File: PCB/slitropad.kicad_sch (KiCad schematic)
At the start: 11 parts, among them SW1 SW_Push, SW2 SW_Push, SW3 SW_Push, SW4 SW_Push, SW5 SW_Push, SW6 SW_Push, SW7 SW_Push, SW8 SW_Push, SW9 SW_Push, U1 XIAO-RP2040-DIP

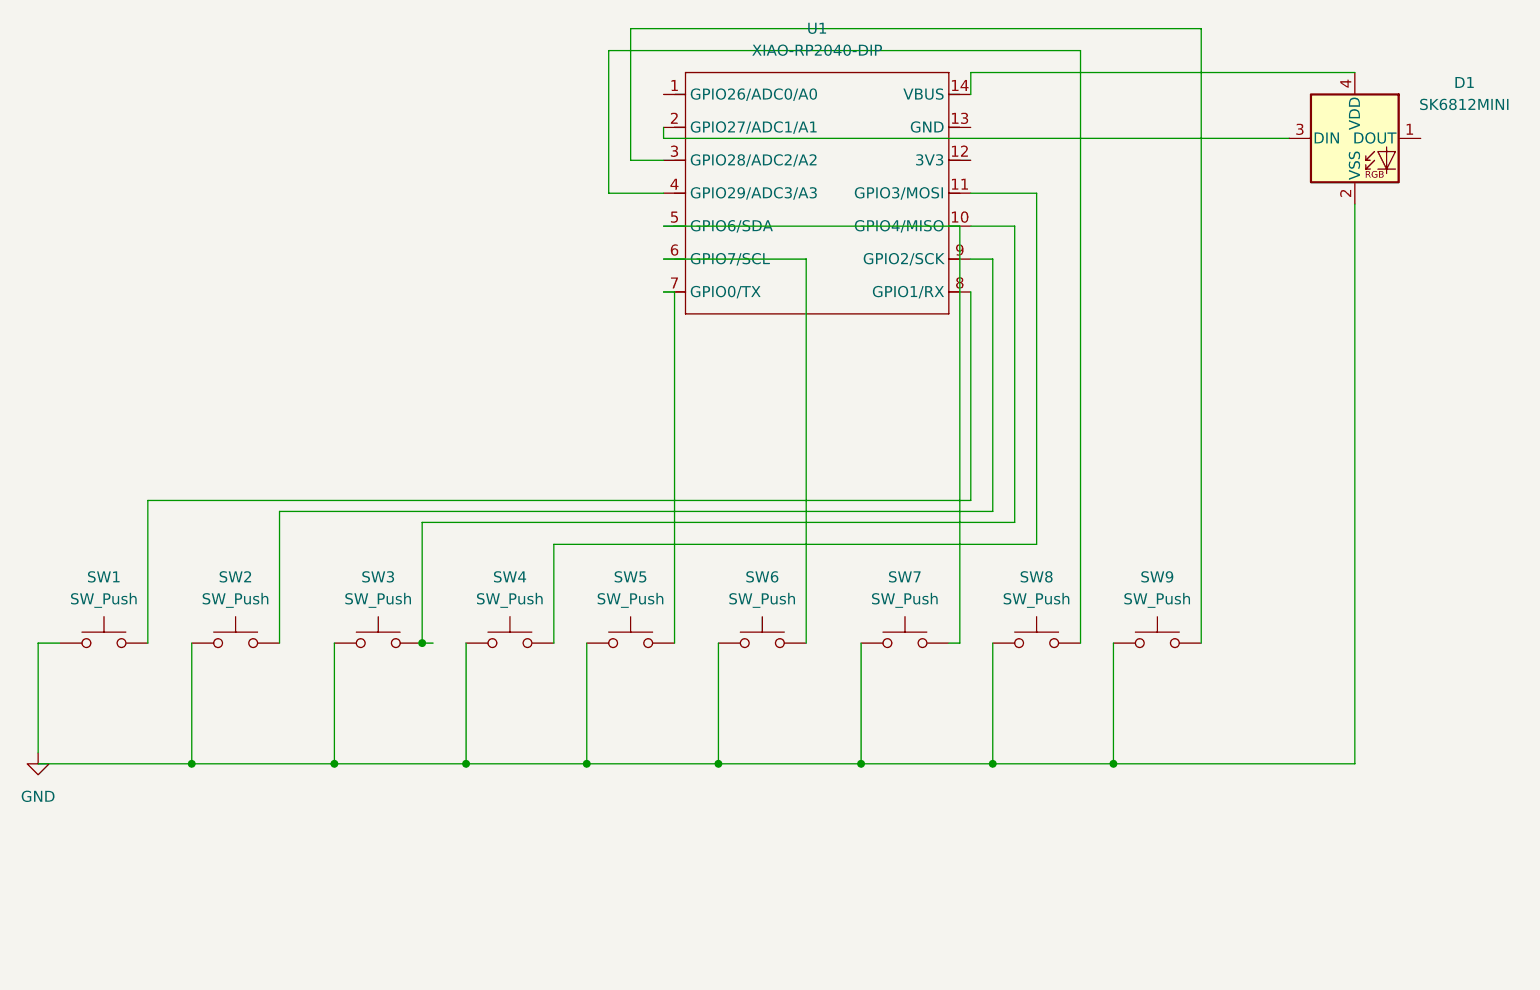
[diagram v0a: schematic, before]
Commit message: push
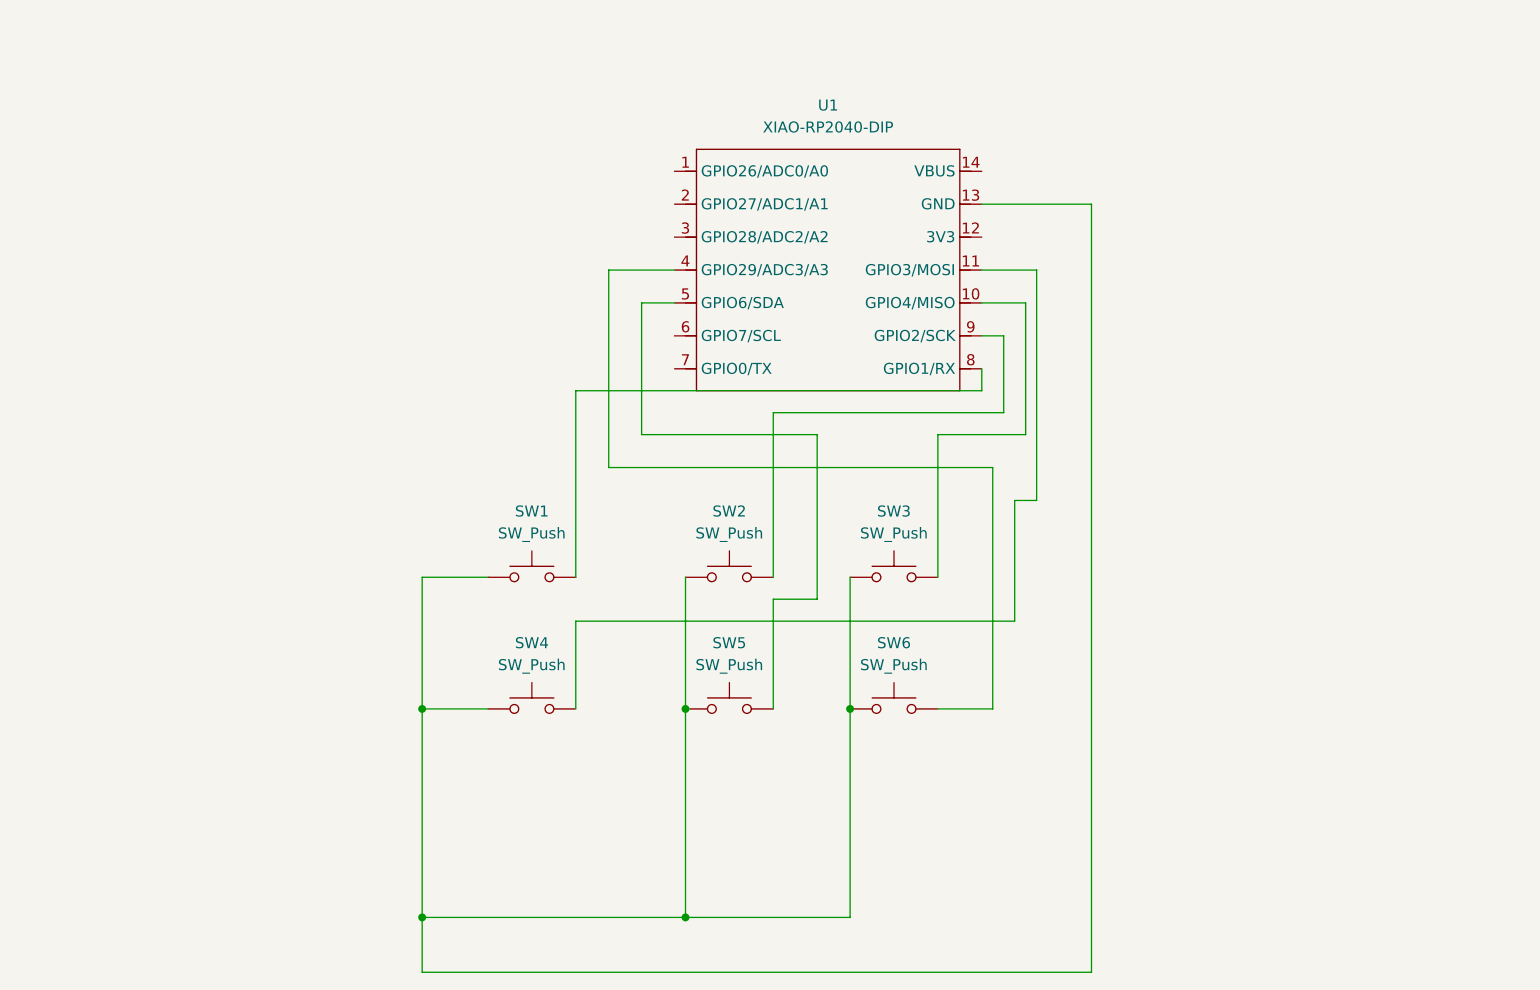
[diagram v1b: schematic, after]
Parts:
- removed D1: SK6812MINI, LED_SMD:LED_SK6812MINI_PLCC4_3.5x3.5mm_P1.75mm, symbol LED:SK6812MINI
- removed SW7, SW8, SW9: SW_Push, Button_Switch_Keyboard:SW_Cherry_MX_1.00u_PCB, symbol Switch:SW_Push
- removed U1: XIAO-RP2040-DIP, footprint:XIAO-RP2040-DIP, symbol Seeed_Studio_XIAO_Series:XIAO-RP2040-DIP
- added U1: XIAO-RP2040-DIP, Xiao Foot:XIAO-RP2040-DIP, symbol Xiao:XIAO-RP2040-DIP
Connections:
- net GND is gone; now on an unnamed net: SW1.1
- net at SW2.1, SW3.1, SW4.1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: now also U1.13 (GND)
- net at SW4.2: now also U1.11 (GPIO3/MOSI)
- net at SW1.2: now also U1.8 (GPIO1/RX)
- net at SW5.2: now also U1.5 (GPIO6/SDA)
- net at SW3.2: now also U1.10 (GPIO4/MISO)
- net at SW6.2: now also U1.4 (GPIO29/ADC3/A3)
- net at SW2.2: now also U1.9 (GPIO2/SCK)
